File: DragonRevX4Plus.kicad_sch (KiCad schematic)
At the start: 5 parts, among them J3 Board Interconnect Female, J4 Conn_02x08_Odd_Even, J5 Video Output Female

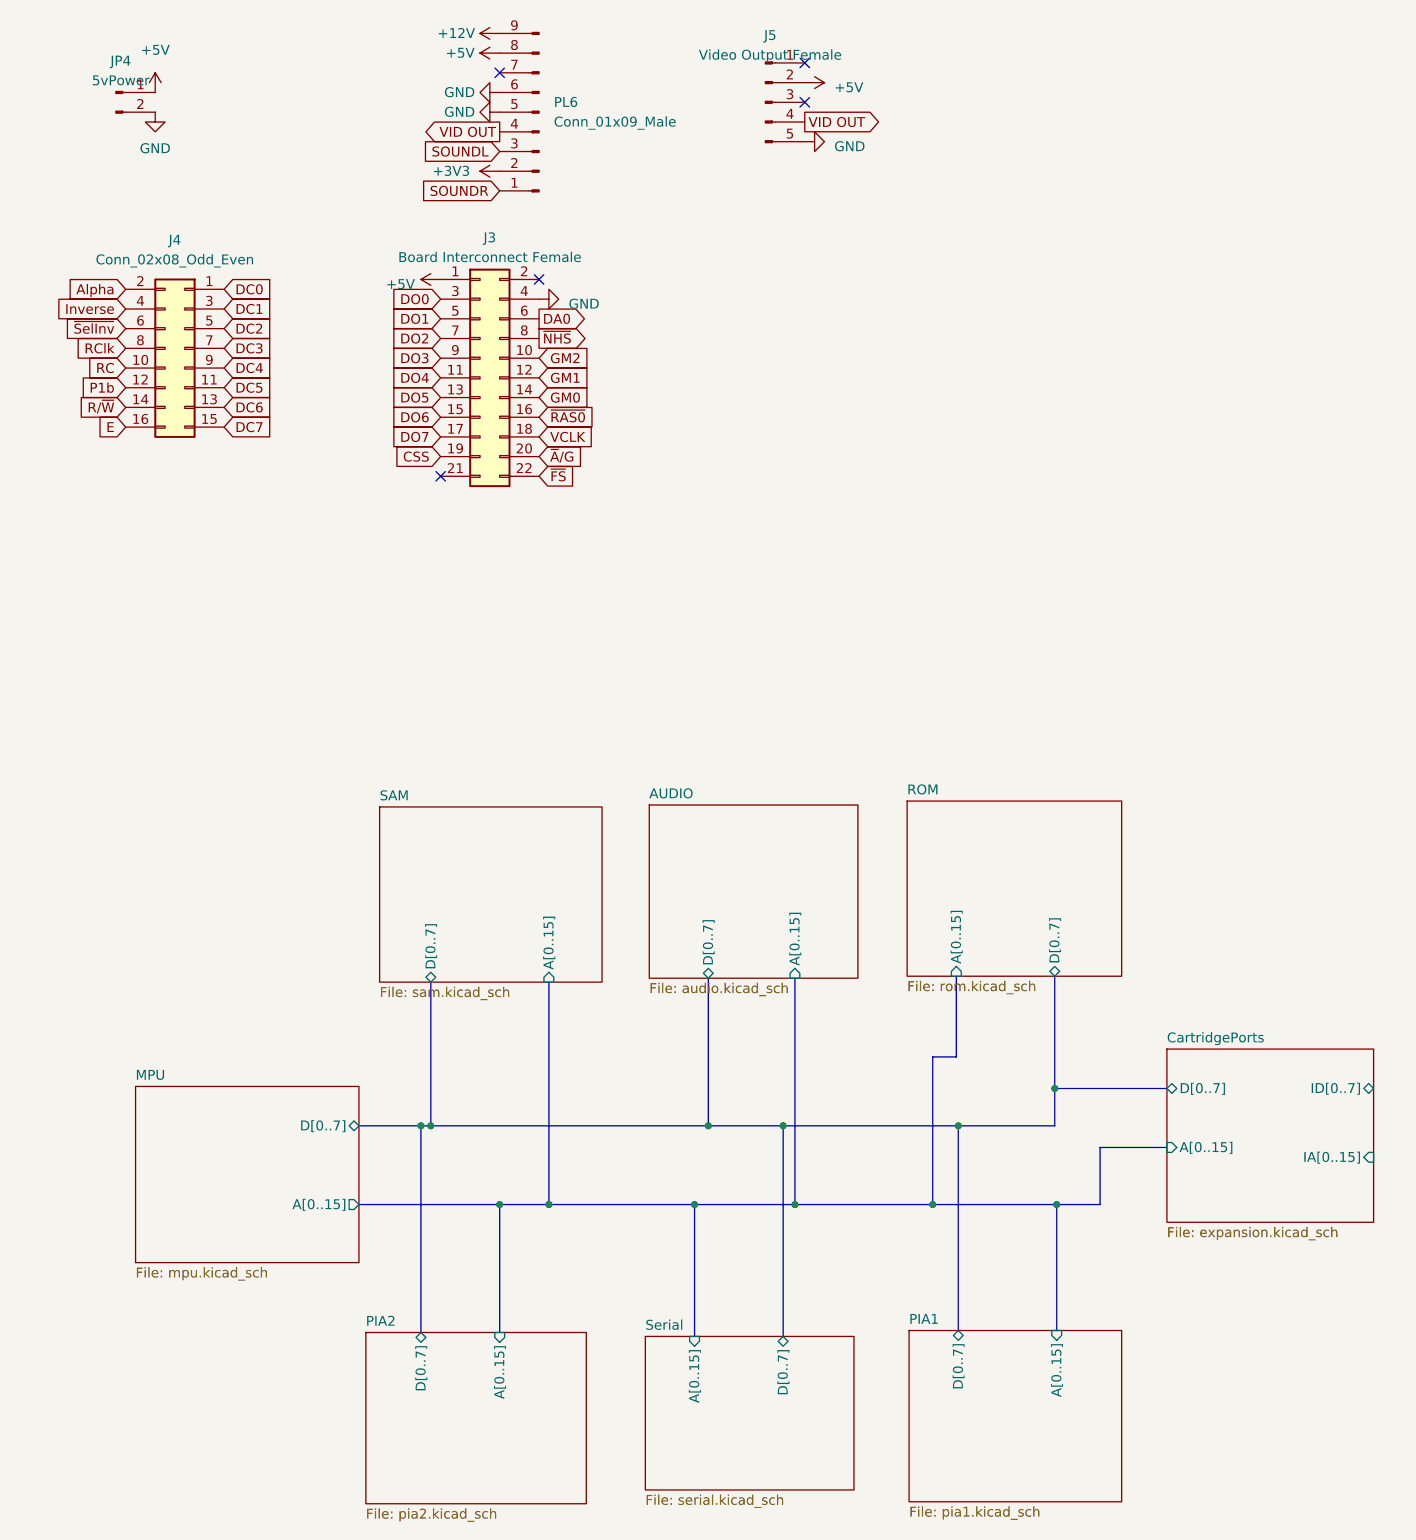
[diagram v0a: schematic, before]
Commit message: Progress routing
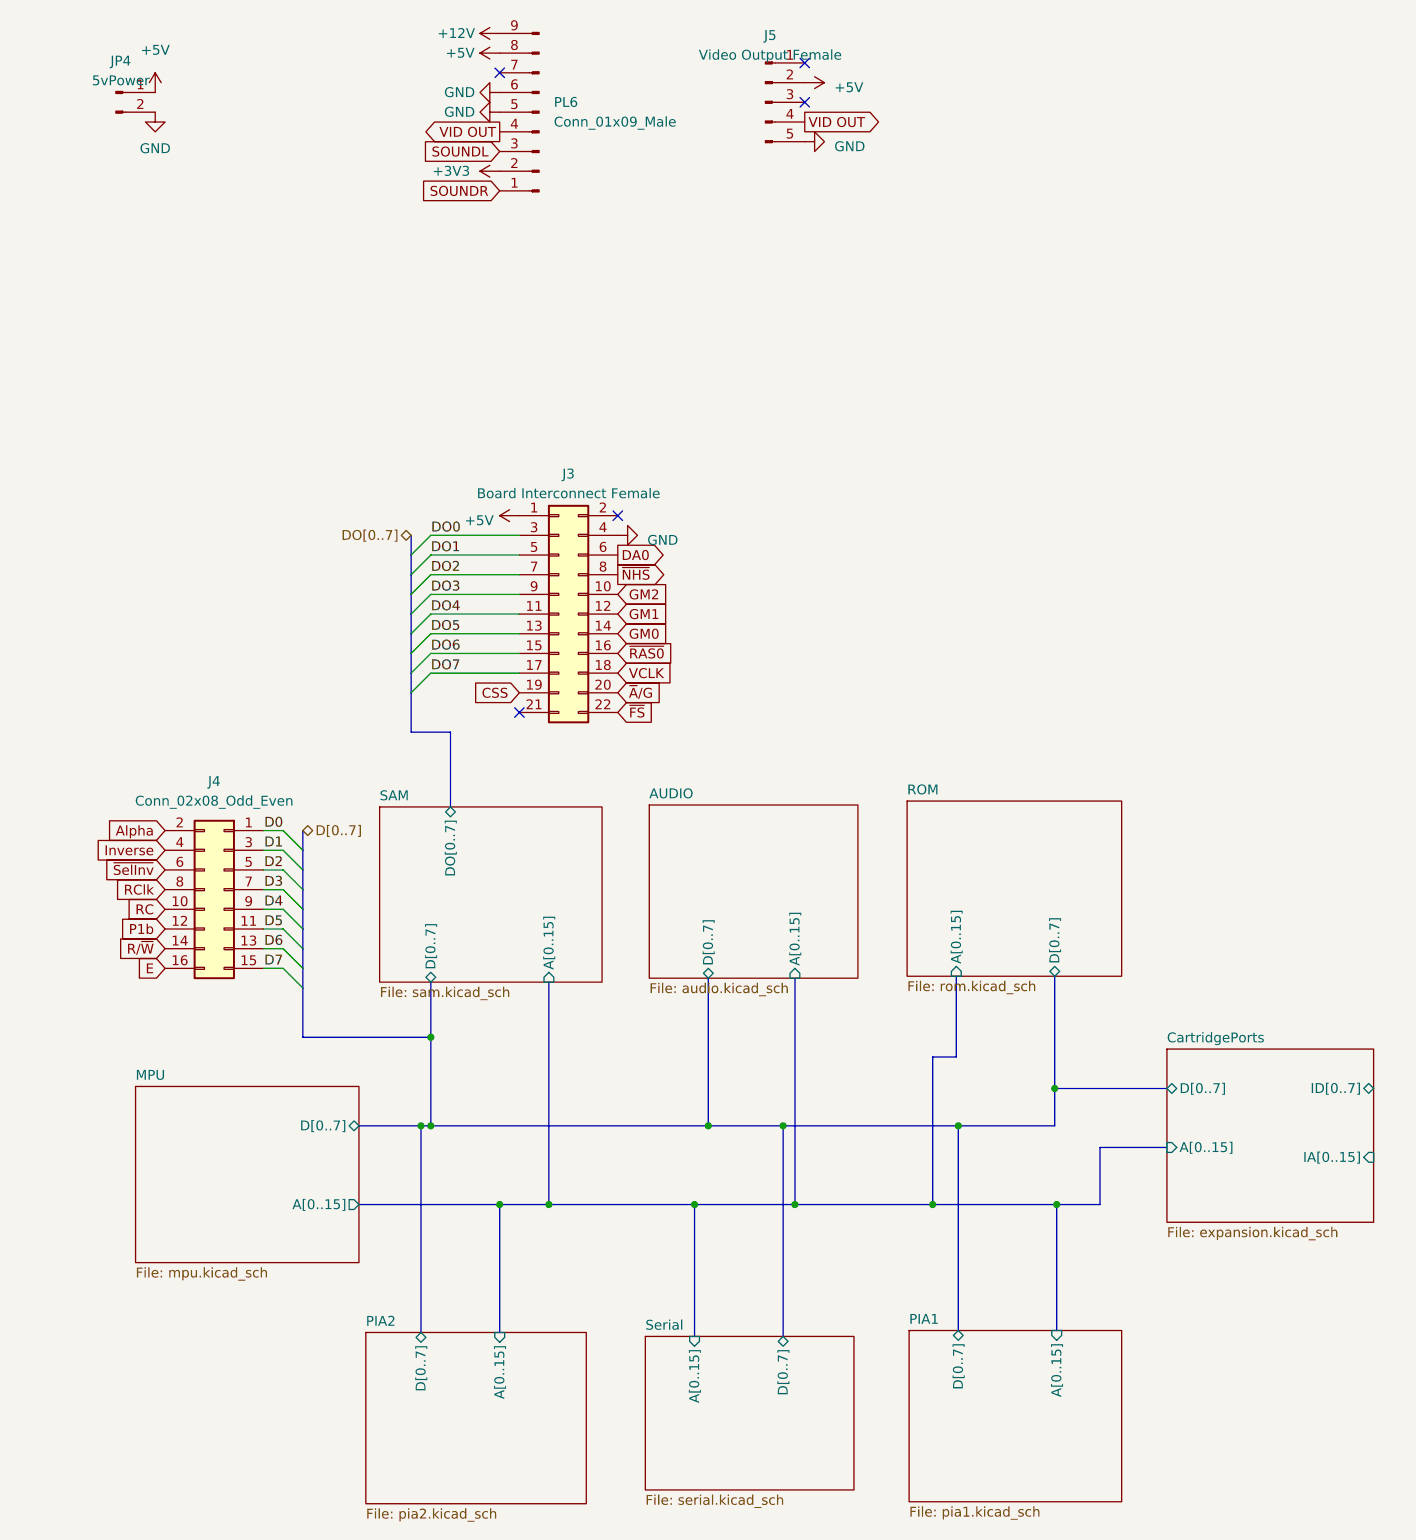
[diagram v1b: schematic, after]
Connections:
- net DC0 renamed D0
- net DC1 renamed D1
- net DC2 renamed D2
- net DC3 renamed D3
- net DC4 renamed D4
- net DC5 renamed D5
- net DC6 renamed D6
- net DC7 renamed D7
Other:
- sheet SAM ports: added DO[0..7]; removed none
- moved on the sheet: J3, J4
